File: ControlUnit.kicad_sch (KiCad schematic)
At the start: 28 parts, among them J4 Conn_01x05_Pin, M1 Motor_DC_ALT, Q1 IRLZ44N, SW1 SW_DPST_x2, SW3 SW_DPST_x2, SW4 SW_SPDT, U3 PIC24HJ128GP502, U5 DRV8871DDA, U6 INA180A1, U7 VL53L0CXV0DH1, Y1 8MHz

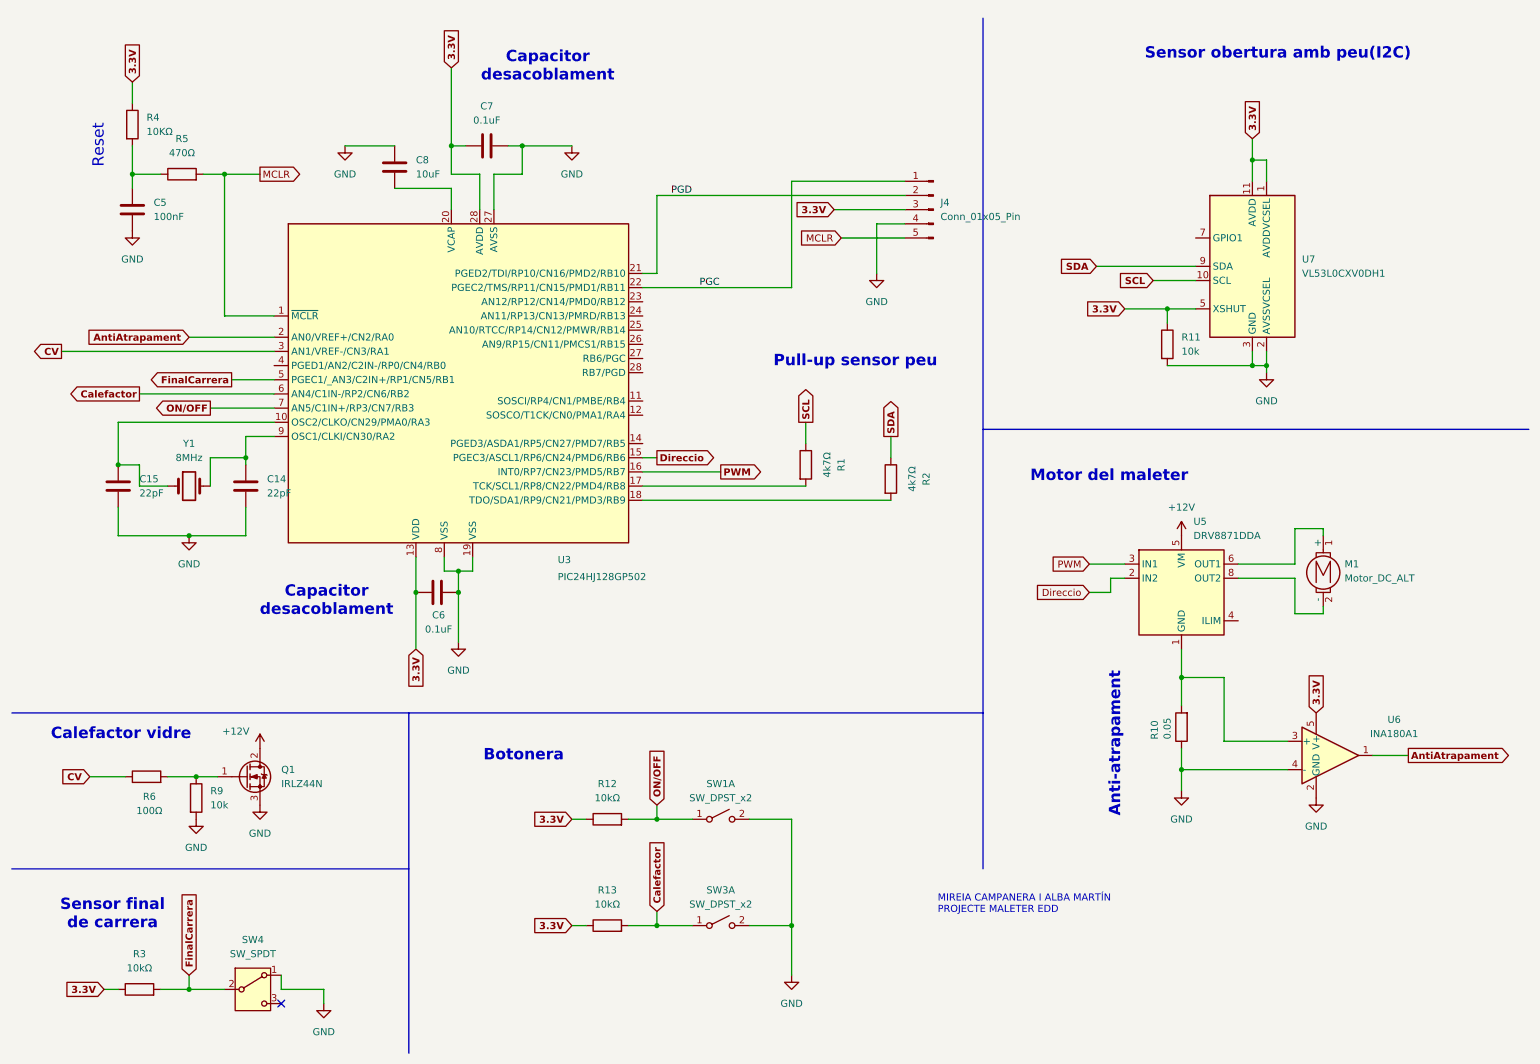
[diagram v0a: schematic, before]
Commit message: Correccions professor
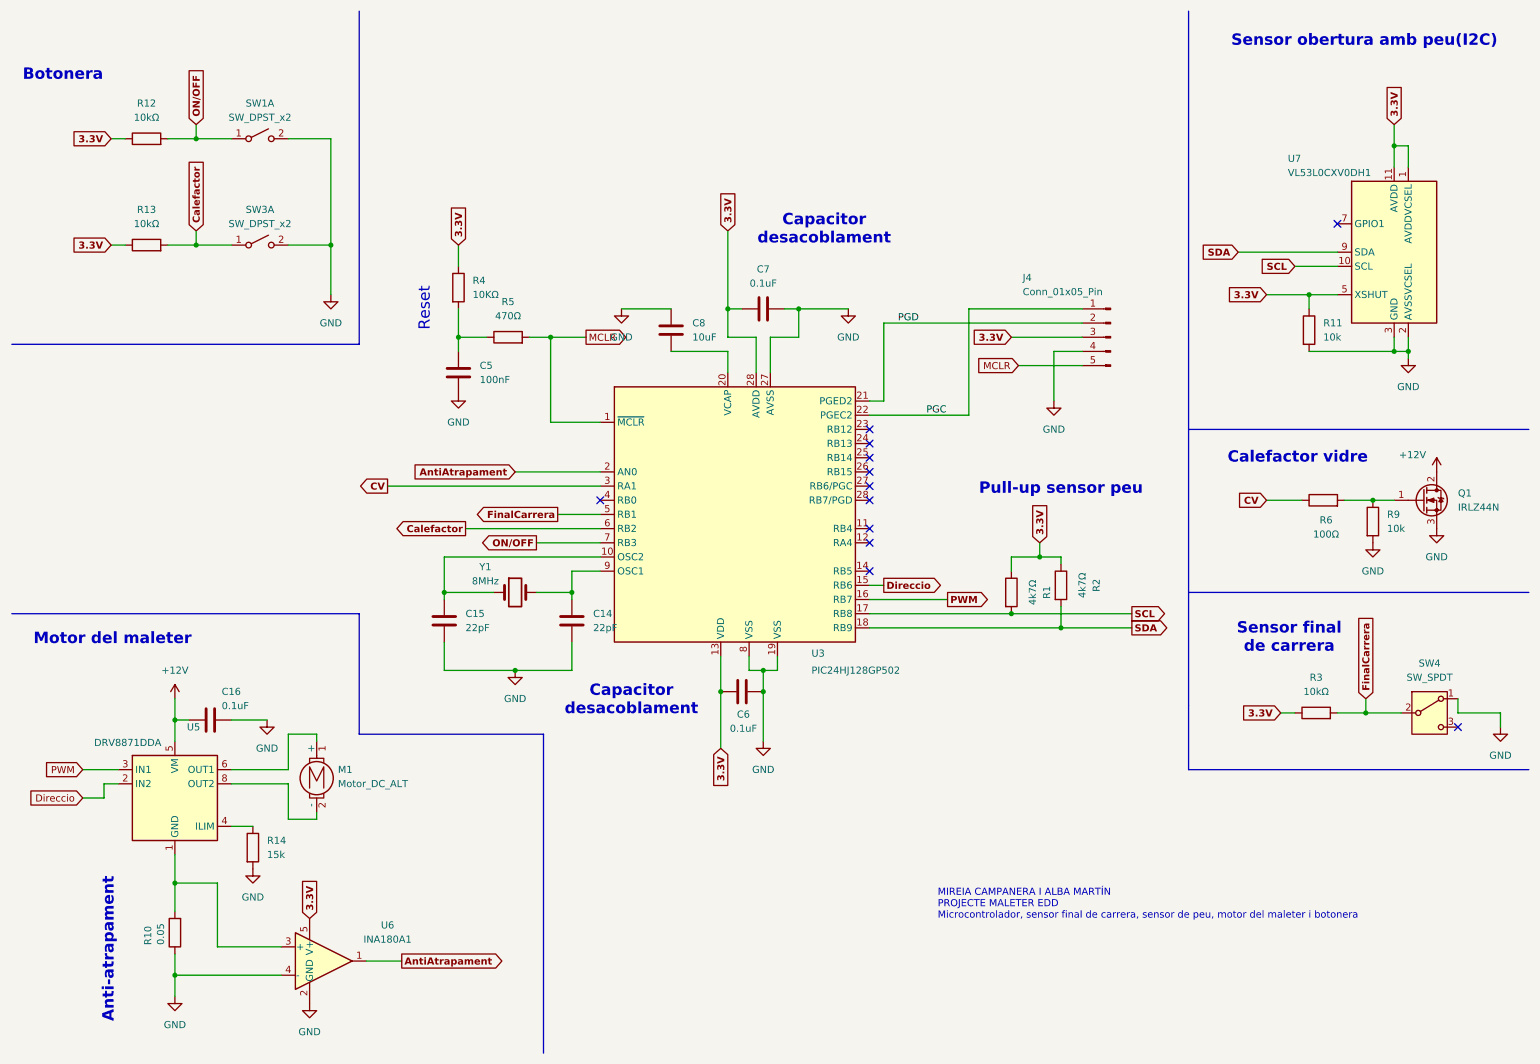
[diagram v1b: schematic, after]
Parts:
- added C16: 0.1uF, Capacitor_SMD:C_0201_0603Metric, symbol Device:C
- added R14: 15k, Resistor_SMD:R_0201_0603Metric, symbol Device:R
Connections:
- net +12V: now also C16.2
- net 3.3V: now also R1.1, R2.1
- net GND: now also C16.1, R14.2
- net SCL: now also R1.2, U3.17 (RB8); no longer R1.1
- net SDA: now also R2.2, U3.18 (RB9); no longer R2.1
- net at U5.4 (ILIM): now also R14.1
- no-connect marks 1 -> 12
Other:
- note added: "MIREIA CAMPANERA I ALBA MARTÍN PROJECTE MALETER EDD Microcontrolador, sensor final de carrera, sensor de peu, motor del maleter i botonera"
- note removed: "MIREIA CAMPANERA I ALBA MARTÍN PROJECTE MALETER EDD"
- moved on the sheet: C14, C15, C5, C6, C7, C8, J4, M1, Q1, R1, R10, R11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
